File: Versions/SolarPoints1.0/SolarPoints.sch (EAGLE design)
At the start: 8 parts, among them Q1 BC548

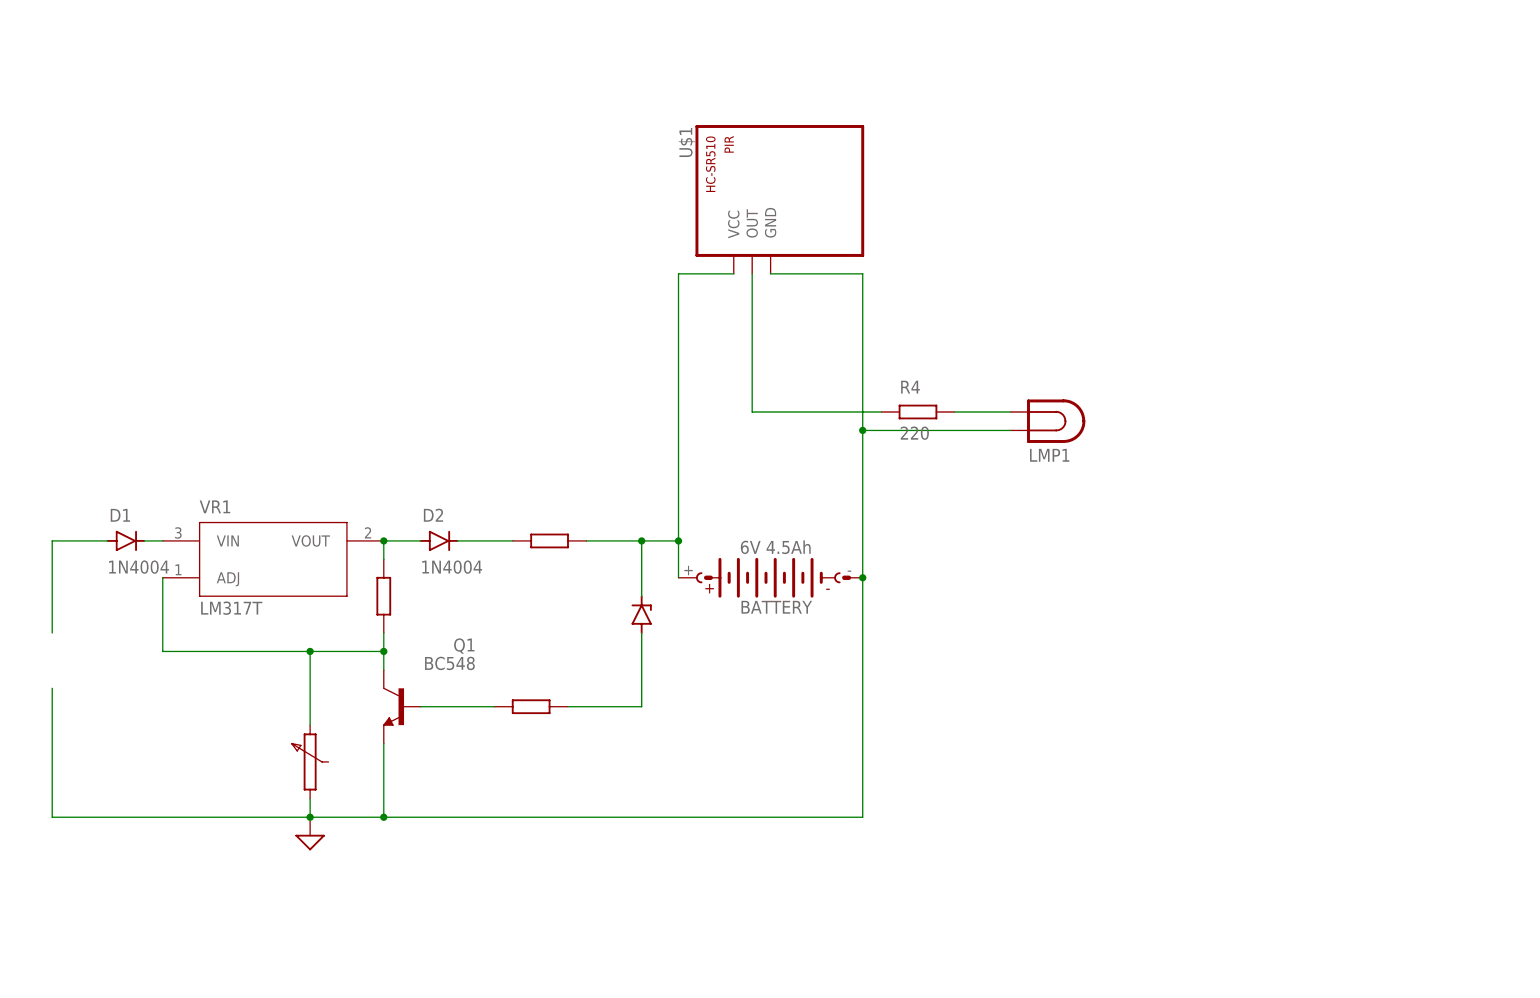
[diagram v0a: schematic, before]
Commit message: Update the finally circuit
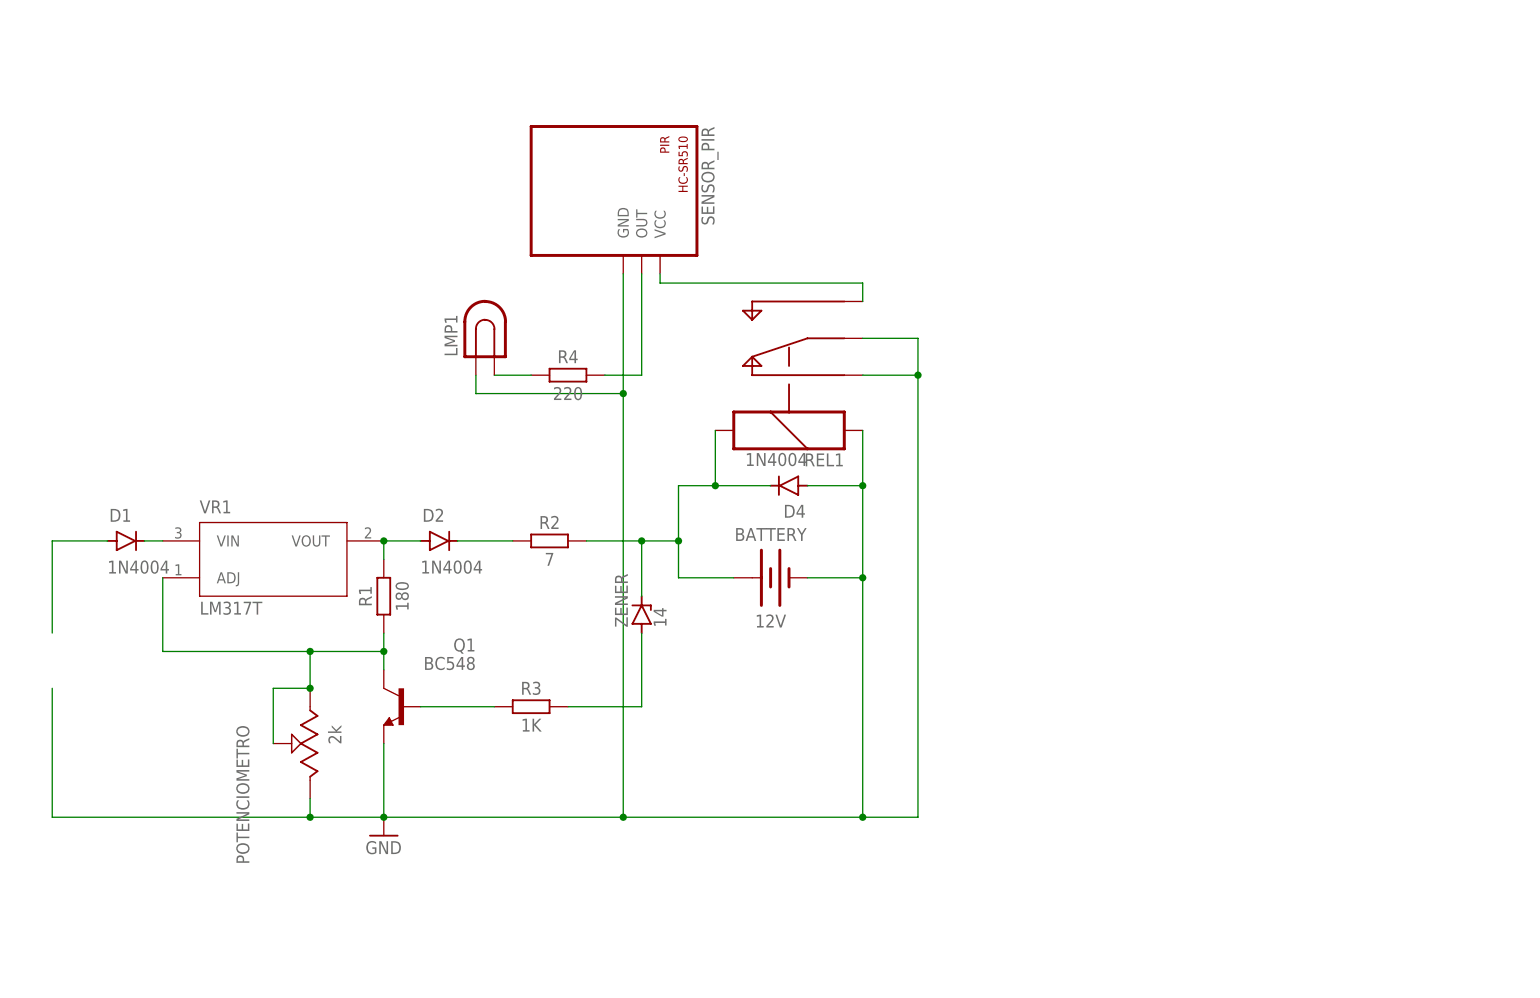
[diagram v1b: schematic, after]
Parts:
- removed U$1: HC-SR501, Sensors_PIR_Lux:HC-SR501
- added D4: 1N4004, Diodes:1N4004
- added POTENCIOMETRO: 2k, Potentiometer_Trimmers:91A1A-B28-B15L
- added R1: 180, Tinkercad:RESISTOR_AXIAL-10.16MM-PITCH
- added R2: 7, Tinkercad:RESISTOR_AXIAL-10.16MM-PITCH
- added R3: 1K, Tinkercad:RESISTOR_AXIAL-10.16MM-PITCH
- added REL1: (no value), special:REL-5PIN
- added SENSOR_PIR: HC-SR501, Sensors_PIR_Lux:HC-SR501
- added ZENER: 14, diode:BZV10
- BATTERY: value 6V 4.5Ah -> 12V; device battery:AB9V -> Tinkercad:BATTERYGENERIC
- R4: device ngspice-simulation:R -> Tinkercad:RESISTOR_AXIAL-10.16MM-PITCH
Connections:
- new net N$12: REL1.O, SENSOR_PIR.VCC
- new net N$2: R3.2, ZENER.A
- net GND: now also D4.A, POTENCIOMETRO.1, REL1.C, REL1.S, REL1.S1, SENSOR_PIR.GND; no longer U$1.GND
- net N$1: now also D4.C, R2.2, REL1.S2, ZENER.C; no longer U$1.VCC
- net N$10: now also R4.2, SENSOR_PIR.OUT; no longer R4.1, U$1.OUT
- net N$3: now also R3.1
- net N$4: now also POTENCIOMETRO.2, POTENCIOMETRO.3, R1.1
- net N$5: now also R1.2
- net N$6: now also R2.1
- net N$7: now also R4.1; no longer R4.2
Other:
- moved on the sheet: LMP1, R4

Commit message: update files
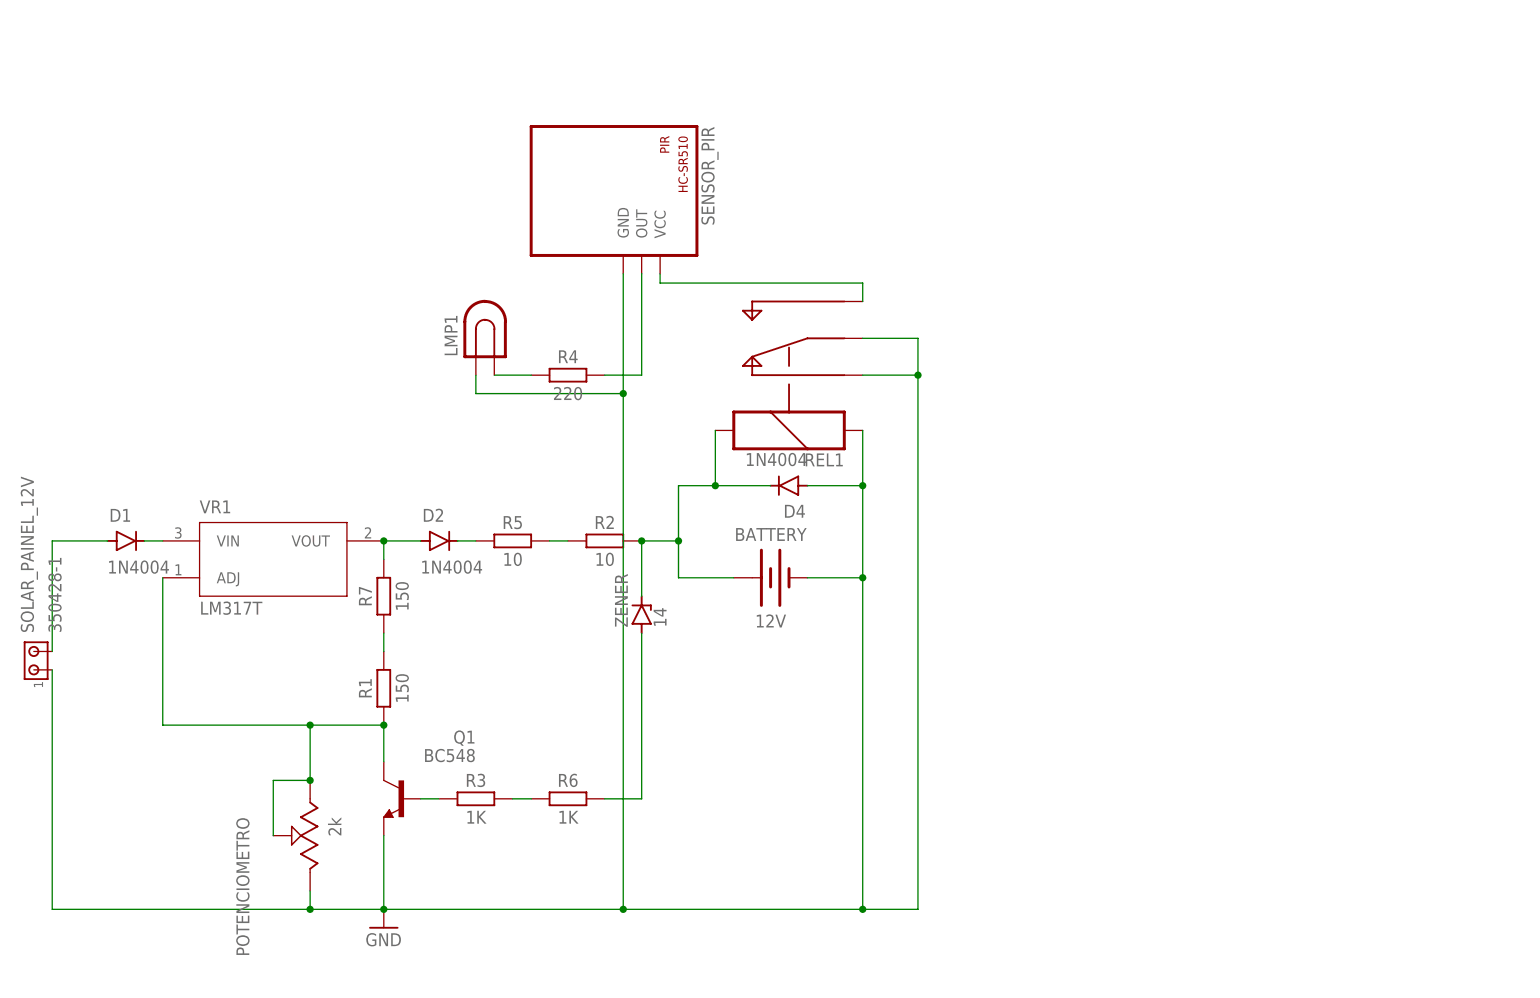
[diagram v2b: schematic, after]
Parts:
- added R5: 10, Tinkercad:RESISTOR_AXIAL-10.16MM-PITCH
- added R6: 1K, Tinkercad:RESISTOR_AXIAL-10.16MM-PITCH
- added R7: 150, Tinkercad:RESISTOR_AXIAL-10.16MM-PITCH
- added SOLAR_PAINEL_12V: 350428-1, con-amp:350428-1
- R1: value 180 -> 150
- R2: value 7 -> 10
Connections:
- new net N$11: R2.1, R5.2
- new net N$13: R3.2, R6.1
- new net N$14: R1.2, R7.1
- net GND: now also SOLAR_PAINEL_12V.1
- net N$2: now also R6.2; no longer R3.2
- net N$5: now also R7.2; no longer R1.2
- net N$6: now also R5.1; no longer R2.1
- net N$8: now also SOLAR_PAINEL_12V.2
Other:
- moved on the sheet: POTENCIOMETRO, Q1, R1, R2, R3

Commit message: update test
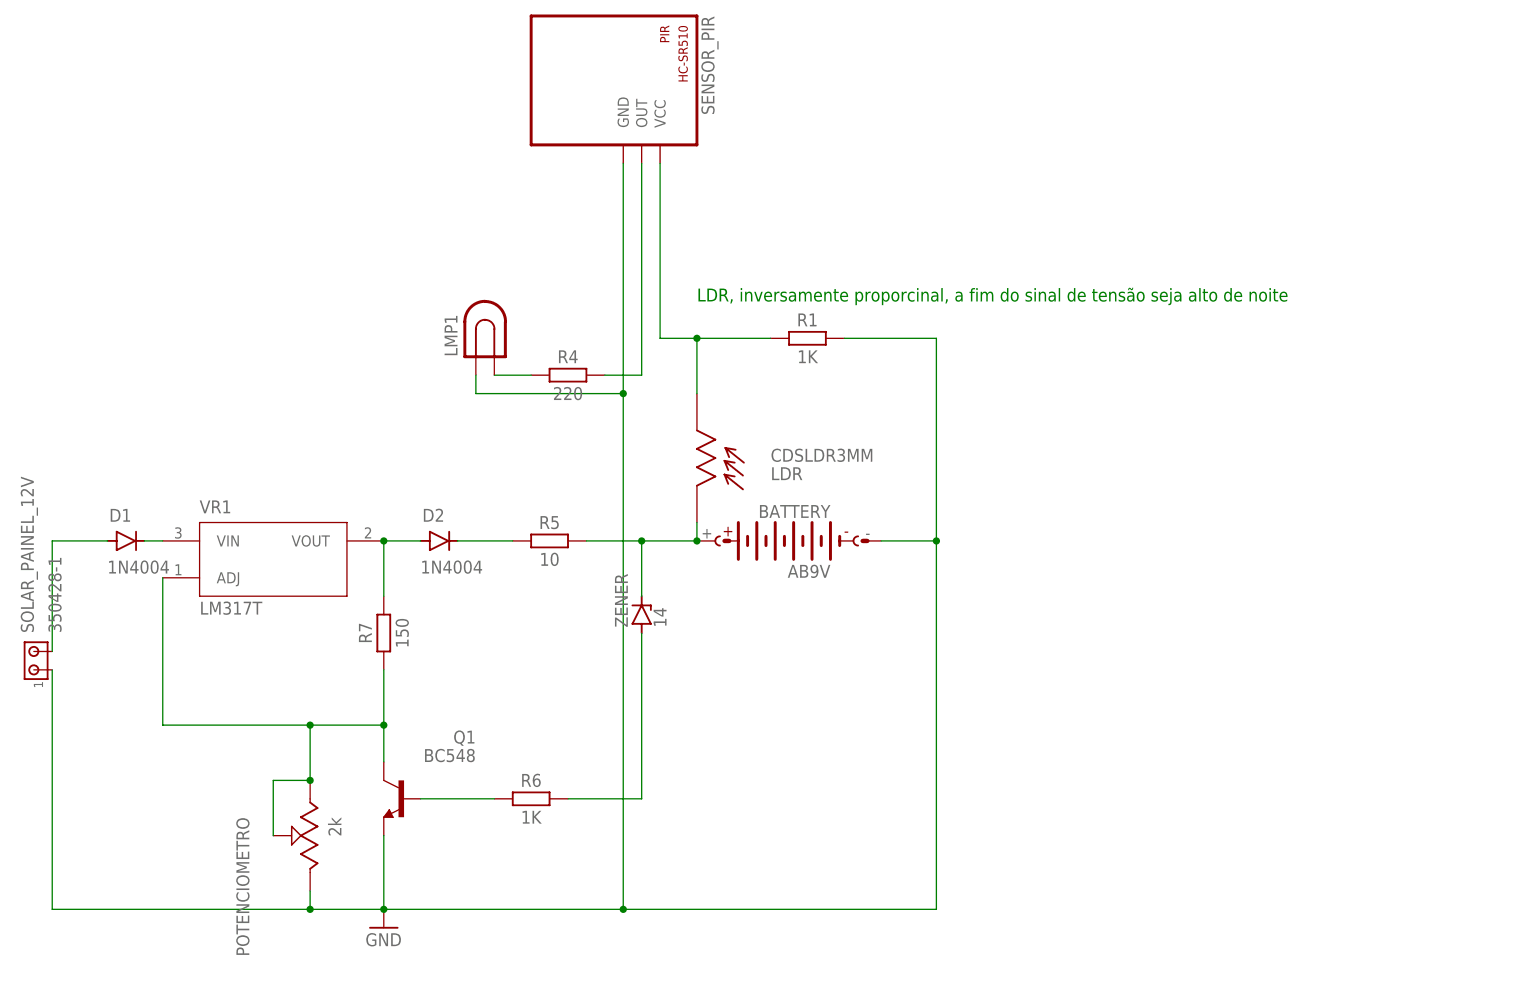
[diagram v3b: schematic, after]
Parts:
- removed D4: 1N4004, Diodes:1N4004
- removed R2: 10, Tinkercad:RESISTOR_AXIAL-10.16MM-PITCH
- removed R3: 1K, Tinkercad:RESISTOR_AXIAL-10.16MM-PITCH
- removed REL1: (no value), special:REL-5PIN
- added LDR: CDSLDR3MM, CEDTv40:CDSLDR3MM
- BATTERY: value 12V -> AB9V; device Tinkercad:BATTERYGENERIC -> battery:AB9V
- R1: value 150 -> 1K
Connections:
- removed net N$11: R2.1, R5.2
- removed net N$13: R3.2, R6.1
- removed net N$14: R1.2, R7.1
- net GND: now also R1.2; no longer D4.A, REL1.C, REL1.S, REL1.S1
- net N$1: now also LDR.P$1, R5.2; no longer D4.C, R2.2, REL1.S2
- net N$12: now also LDR.P$2, R1.1; no longer REL1.O
- net N$3: now also R6.1; no longer R3.1
- net N$4: now also R7.1; no longer R1.1
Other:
- note added: "LDR, inversamente proporcinal, a fim do sinal de tensão seja alto de noite"
- moved on the sheet: R1, R5, R6, R7, SENSOR_PIR
